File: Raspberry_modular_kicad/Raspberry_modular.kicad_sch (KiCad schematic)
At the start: 21 parts, among them J1 Raspberry_Pi_2_3, U1 MCP3008, U3 MCP3008

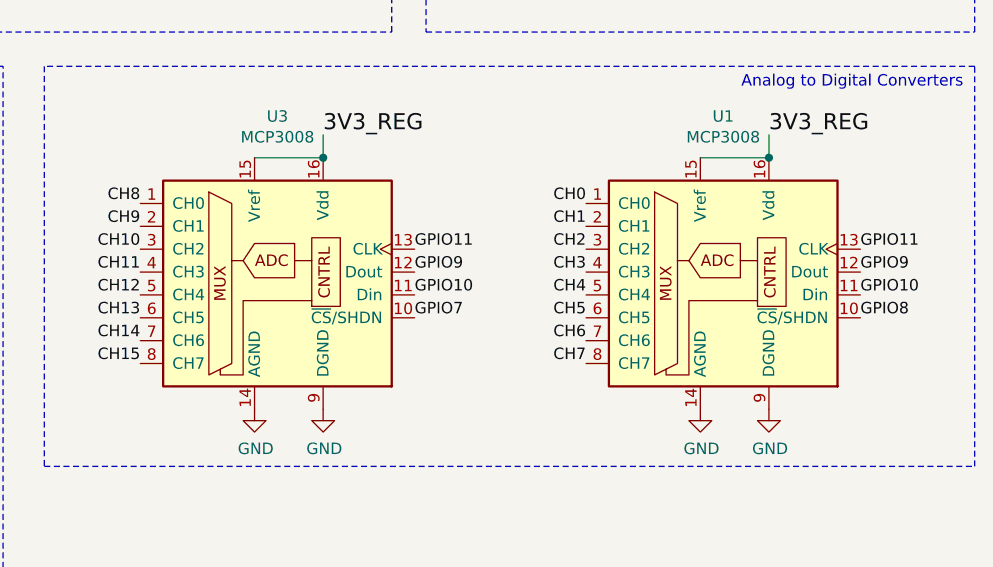
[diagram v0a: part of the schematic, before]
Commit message: [FIX] Production build
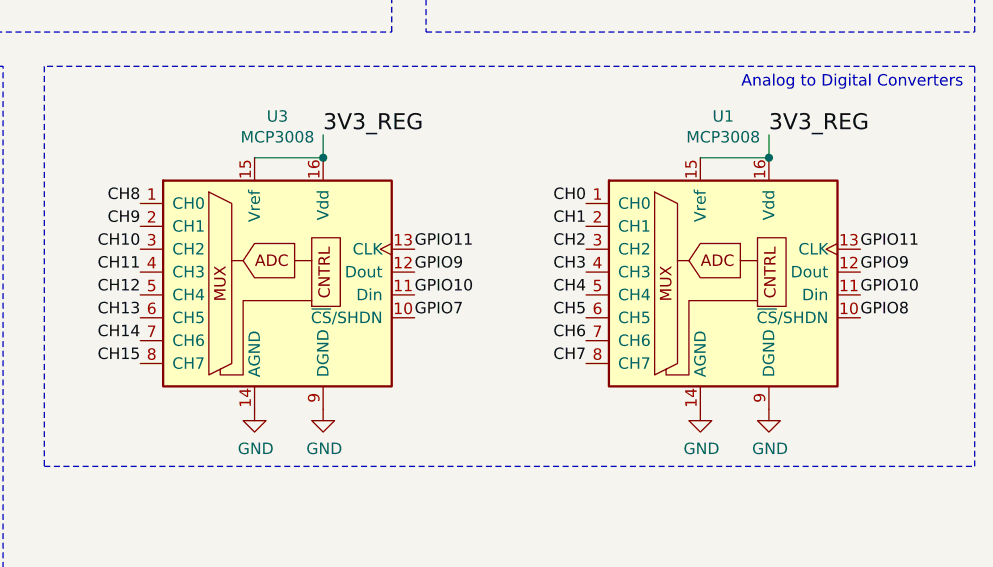
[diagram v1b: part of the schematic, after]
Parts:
- U1, U3: JLCPCB Position Offset (none) -> 0.65, 0; JLCPCB Rotation Offset (none) -> 270
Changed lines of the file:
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@@
+      (effects (font (size 1.27 1.27)) hide)
+    )
+    (property "JLCPCB Rotation Offset" "270" (at 273.05 172.72 0)
+      (effects (font (size 1.27 1.27)) hide)
+    )
+    (property "JLCPCB Position Offset" "0.65, 0" (at 273.05 172.72 0)
       (effects (font (size 1.27 1.27)) hide)
     )
@@
       (effects (font (size 1.27 1.27)) hide)
     )
+    (property "JLCPCB Rotation Offset" "270" (at 223.52 172.72 0)
+      (effects (font (size 1.27 1.27)) hide)
+    )
+    (property "JLCPCB Position Offset" "0.65, 0" (at 223.52 172.72 0)
+      (effects (font (size 1.27 1.27)) hide)
+    )
